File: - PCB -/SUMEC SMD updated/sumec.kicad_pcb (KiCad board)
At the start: 2 copper layers, 92 x 56.5 mm, 59 parts, among them IC1 XT30U-F, J1 Conn_01x04_Pin, J2 Conn_01x01_Pin, J3 Conn_01x03_Pin, J4 Conn_01x02, J5 TYPE-C-31-M-12, J6 Conn_01x06_Pin, J7 Conn_01x06_Pin, J8 TSOP382xx, J9 Conn_01x06_Pin, SW1 SW_Push, SW2 SW_Push, SW3 SW_Push, U1 TB6612FNG, U2 ESP32-S3-WROOM-1, U3 USBLC6-2SC6, U4 QRE1113, U5 QRE1113, U6 QRE1113, U7 LM1084IS-5.0/NOPB, U8 LM1084IS-3.3/NOPB

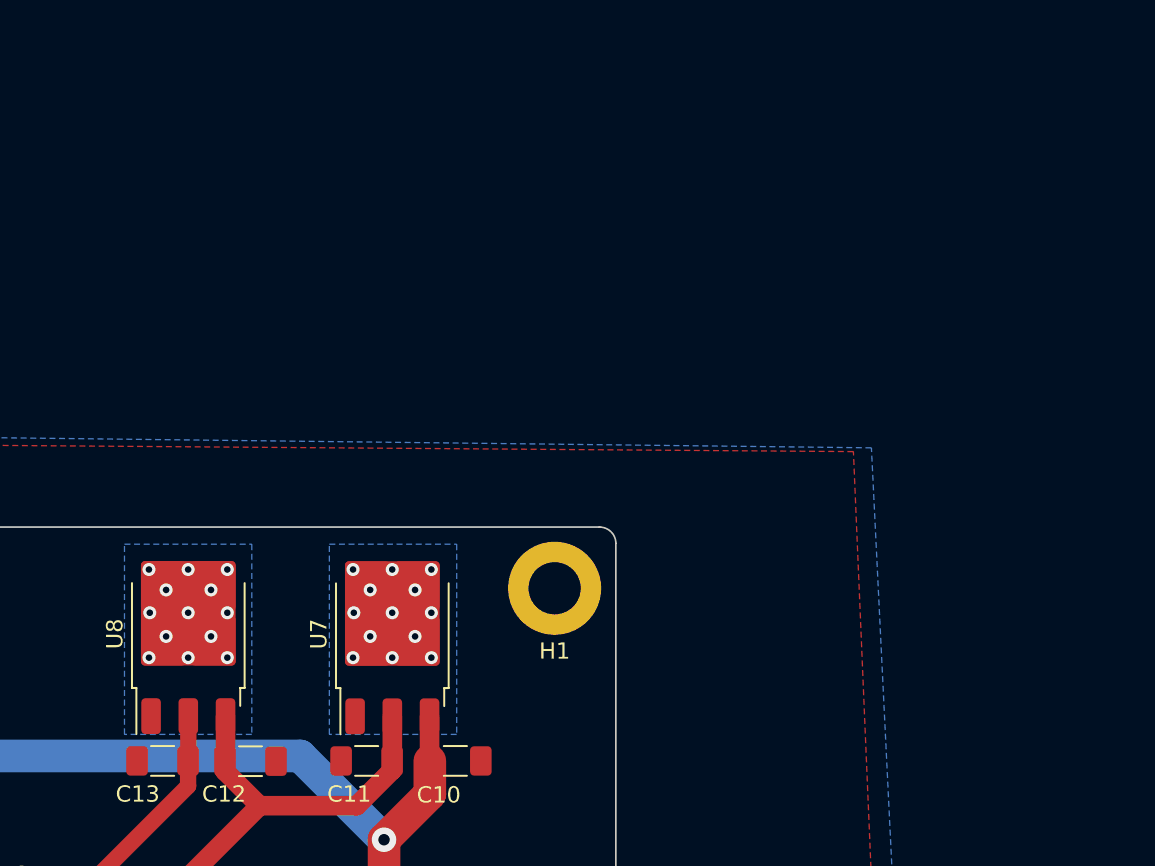
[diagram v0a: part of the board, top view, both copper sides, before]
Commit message: cleanup sumec enchanced
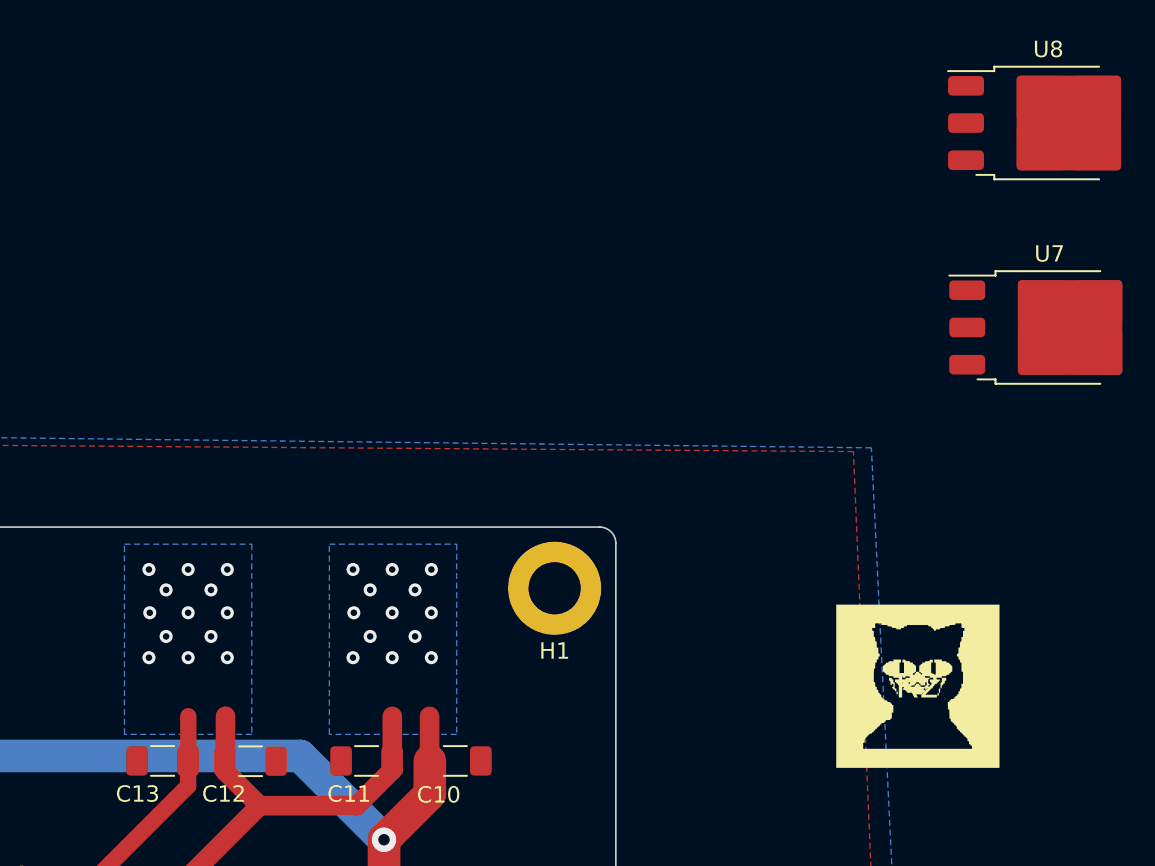
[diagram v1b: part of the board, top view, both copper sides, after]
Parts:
- added R2: R, sumec-smd_library:car cool smol, F.Cu at (261.2, 54.2)
- moved U8 61.3 mm to (269.2, 19.8), turned to 0 degrees
- moved U7 44.4 mm to (269.3, 32.3), turned to 0 degrees
